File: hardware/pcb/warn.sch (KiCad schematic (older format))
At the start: 17 parts, among them CON2 MMCX_CONN, Q1 BSS138, U10 BU4SU69G2, U11 BU4SU69G2, U12 NC7WZ17, U9 TPS61041

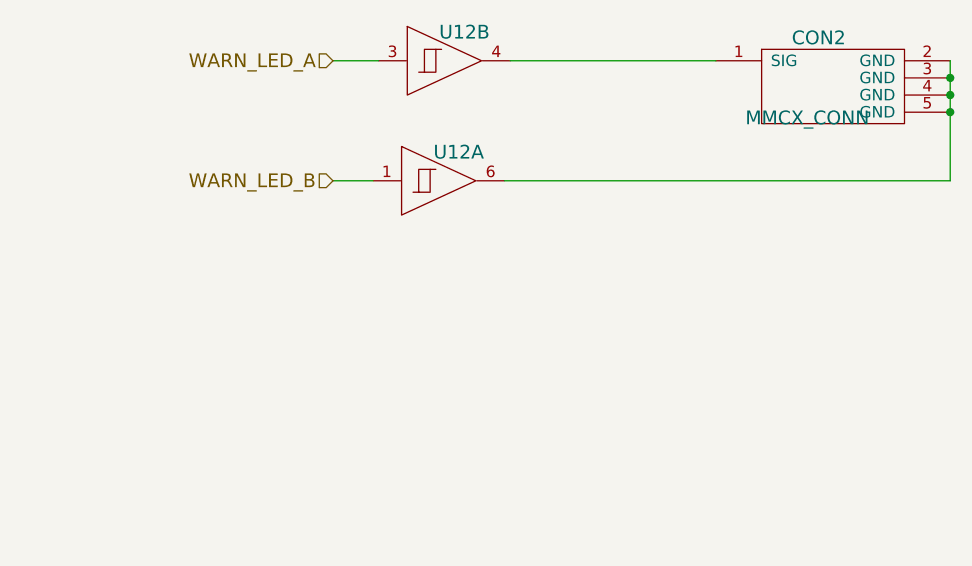
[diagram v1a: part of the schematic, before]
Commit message: pre-net import
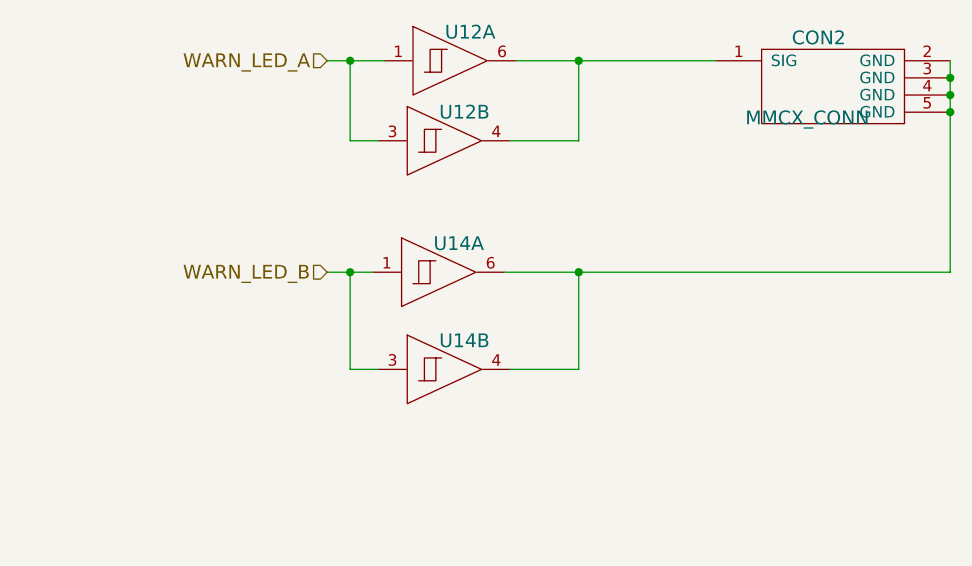
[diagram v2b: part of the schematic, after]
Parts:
- added U14: NC7WZ17, Housings_SOT-23_SOT-143_TSOT-6:SC-70-6, symbol NC7WZ17
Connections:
- net +3V: now also U14.5 (+3V), U14.5 (+3V)
- net GND: now also U14.2 (GND), U14.2 (GND)
- net WARN_LED_A: now also U12.1
- net WARN_LED_B: now also U14.1, U14.3; no longer U12.1
- net at CON2.1 (SIG), U12.4: now also U12.6
- net at CON2.2 (GND), CON2.3 (GND), CON2.4 (GND)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: now also U14.4, U14.6; no longer U12.6
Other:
- moved on the sheet: U12A, U12B
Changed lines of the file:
@@
 Text HLabel 5675 5650 0    60   Input ~ 0
 PIEZO_OUT
-Text HLabel 7975 2575 0    60   Input ~ 0
+Text HLabel 7950 2575 0    60   Input ~ 0
 WARN_LED_A
-Text HLabel 7975 3100 0    60   Input ~ 0
+Text HLabel 7950 3500 0    60   Input ~ 0
 WARN_LED_B
 Text HLabel 1700 2800 0    60   Input ~ 0
@@
 EN needs to be at least\n1.2v
 $Comp
-L MMCX_CONN CON2
-U 1 1 5540F4C0
-P 9900 2675
-F 0 "CON2" H 10100 2875 60  0000 C CNN
-F 1 "MMCX_CONN" H 10050 2525 60  0000 C CNN
-F 2 "aero:CONMMCX002-SMD" H 9900 2675 60  0001 C CNN
-F 3 "" H 9900 2675 60  0000 C CNN
-	1    9900 2675
-	1    0    0    -1
-$EndComp
-$Comp
 L PIEZO AUD1
 U 1 1 554BE33E
@@
 L NC7WZ17 U12
 U 1 1 55B160CF
-P 8425 3100
-F 0 "U12" H 8525 3225 60  0000 C CNN
-F 1 "NC7WZ17" H 8600 2925 60  0001 C CNN
-F 2 "Housings_SOT-23_SOT-143_TSOT-6:SC-70-6" H 8425 3100 60  0001 C CNN
-F 3 "" H 8425 3100 60  0000 C CNN
-	1    8425 3100
+P 8475 2575
+F 0 "U12" H 8575 2700 60  0000 C CNN
+F 1 "NC7WZ17" H 8650 2400 60  0001 C CNN
+F 2 "Housings_SOT-23_SOT-143_TSOT-6:SC-70-6" H 8475 2575 60  0001 C CNN
+F 3 "" H 8475 2575 60  0000 C CNN
+	1    8475 2575
 	1    0    0    -1
 $EndComp
@@
 L NC7WZ17 U12
 U 2 1 55B161A1
-P 8450 2575
-F 0 "U12" H 8550 2700 60  0000 C CNN
-F 1 "NC7WZ17" H 8625 2400 60  0001 C CNN
-F 2 "Housings_SOT-23_SOT-143_TSOT-6:SC-70-6" H 8450 2575 60  0001 C CNN
-F 3 "" H 8450 2575 60  0000 C CNN
-	2    8450 2575
+P 8450 2925
+F 0 "U12" H 8550 3050 60  0000 C CNN
+F 1 "NC7WZ17" H 8625 2750 60  0001 C CNN
+F 2 "Housings_SOT-23_SOT-143_TSOT-6:SC-70-6" H 8450 2925 60  0001 C CNN
+F 3 "" H 8450 2925 60  0000 C CNN
+	2    8450 2925
 	1    0    0    -1
 $EndComp
@@
 Wire Wire Line
 	2350 2800 2700 2800
-Wire Wire Line
-	10675 2575 10675 3100
 Connection ~ 10675 2650
 Connection ~ 10675 2725
@@
 	5675 5650 5875 5650
 Wire Wire Line
-	8150 3100 7975 3100
-Wire Wire Line
-	7975 2575 8175 2575
-Wire Wire Line
-	8750 2575 9650 2575
-Wire Wire Line
-	10675 3100 8725 3100
-Wire Wire Line
 	3900 4725 6225 4725
+$Comp
+L NC7WZ17 U14
+U 1 1 561D6D8E
+P 8425 3500
+F 0 "U14" H 8525 3625 60  0000 C CNN
+F 1 "NC7WZ17" H 8600 3325 60  0001 C CNN
+F 2 "Housings_SOT-23_SOT-143_TSOT-6:SC-70-6" H 8425 3500 60  0001 C CNN
+F 3 "" H 8425 3500 60  0000 C CNN
+	1    8425 3500
+	1    0    0    -1
+$EndComp
+$Comp
+L NC7WZ17 U14
+U 2 1 561D6E0B
+P 8450 3925
+F 0 "U14" H 8550 4050 60  0000 C CNN
+F 1 "NC7WZ17" H 8625 3750 60  0001 C CNN
+F 2 "Housings_SOT-23_SOT-143_TSOT-6:SC-70-6" H 8450 3925 60  0001 C CNN
+F 3 "" H 8450 3925 60  0000 C CNN
+	2    8450 3925
+	1    0    0    -1
+$EndComp
+$Comp
+L MMCX_CONN CON2
+U 1 1 5540F4C0
+P 9900 2675
+F 0 "CON2" H 10100 2875 60  0000 C CNN
+F 1 "MMCX_CONN" H 10050 2525 60  0000 C CNN
+F 2 "aero:CONMMCX002-SMD" H 9900 2675 60  0001 C CNN
+F 3 "" H 9900 2675 60  0000 C CNN
+	1    9900 2675
+	1    0    0    -1
+$EndComp
+Wire Wire Line
+	7950 2575 8200 2575
+Wire Wire Line
+	8175 2925 8050 2925
+Wire Wire Line
+	8050 2925 8050 2575
+Connection ~ 8050 2575
+Wire Wire Line
+	8775 2575 9650 2575
+Wire Wire Line
+	8750 2925 9050 2925
+Wire Wire Line
+	9050 2925 9050 2575
+Connection ~ 9050 2575
+Wire Wire Line
+	7950 3500 8150 3500
+Wire Wire Line
+	8050 3500 8050 3925
+Wire Wire Line
+	8050 3925 8175 3925
+Connection ~ 8050 3500
+Wire Wire Line
+	10675 3500 8725 3500
+Wire Wire Line
+	10675 2575 10675 3500
+Wire Wire Line
+	8750 3925 9050 3925
+Wire Wire Line
+	9050 3925 9050 3500
+Connection ~ 9050 3500
 $EndSCHEMATC
